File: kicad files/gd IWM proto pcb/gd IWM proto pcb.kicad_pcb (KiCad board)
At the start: 2 copper layers, 93.8 x 65.4 mm, 60 parts, among them J1 DB19_4, J10 CPx_LA, J11 Addr_Main_Data, J13 Game Port, J14 CTRL2, J15 IWM-LA, J16 FDC Hdr, J17 EN, J18 CTRL1, J19 Slot_Maker, J2 DSUB19, J3 DB19_16, J4 EN, J5 EN, J6 PWR, J8 555_LA, U1 NE556, U2 NE556, U3 IWM, U4 HCT251

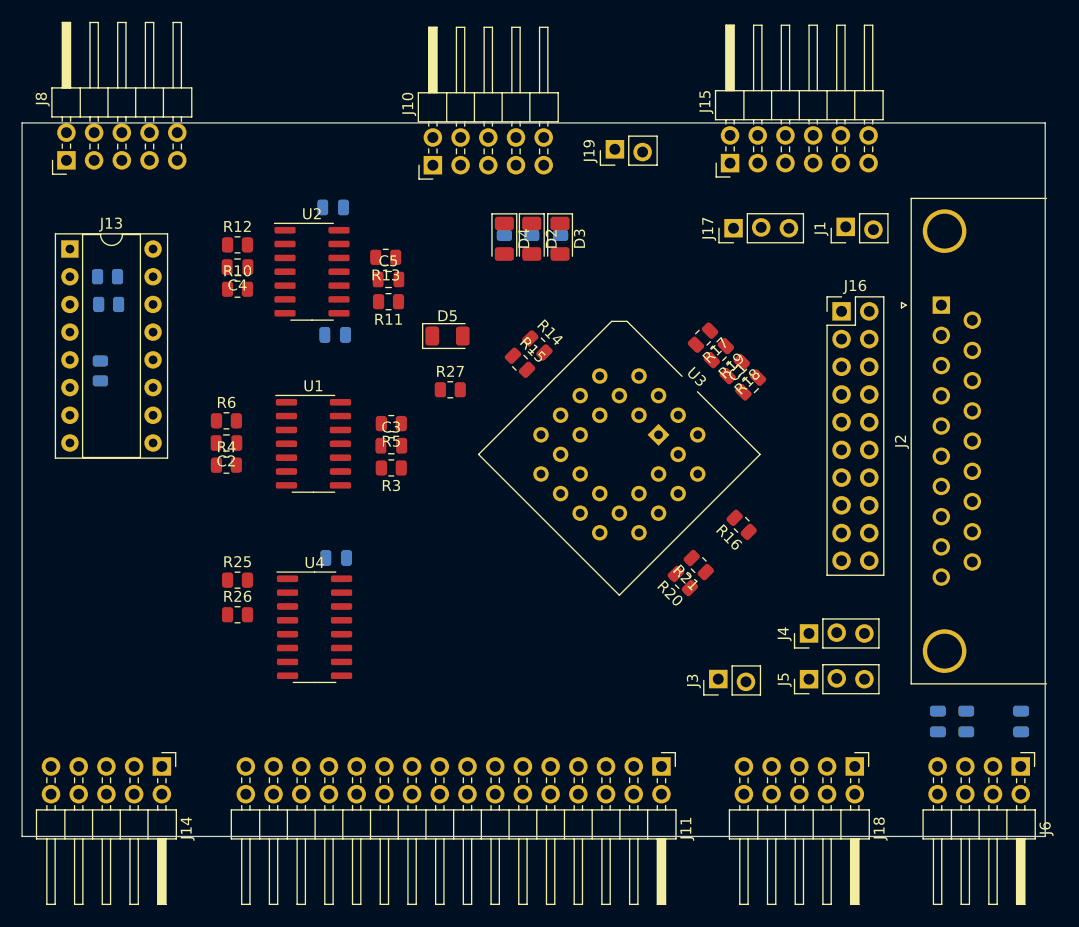
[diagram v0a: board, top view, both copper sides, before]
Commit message: routed most of critical signals. now trying to get LA headers
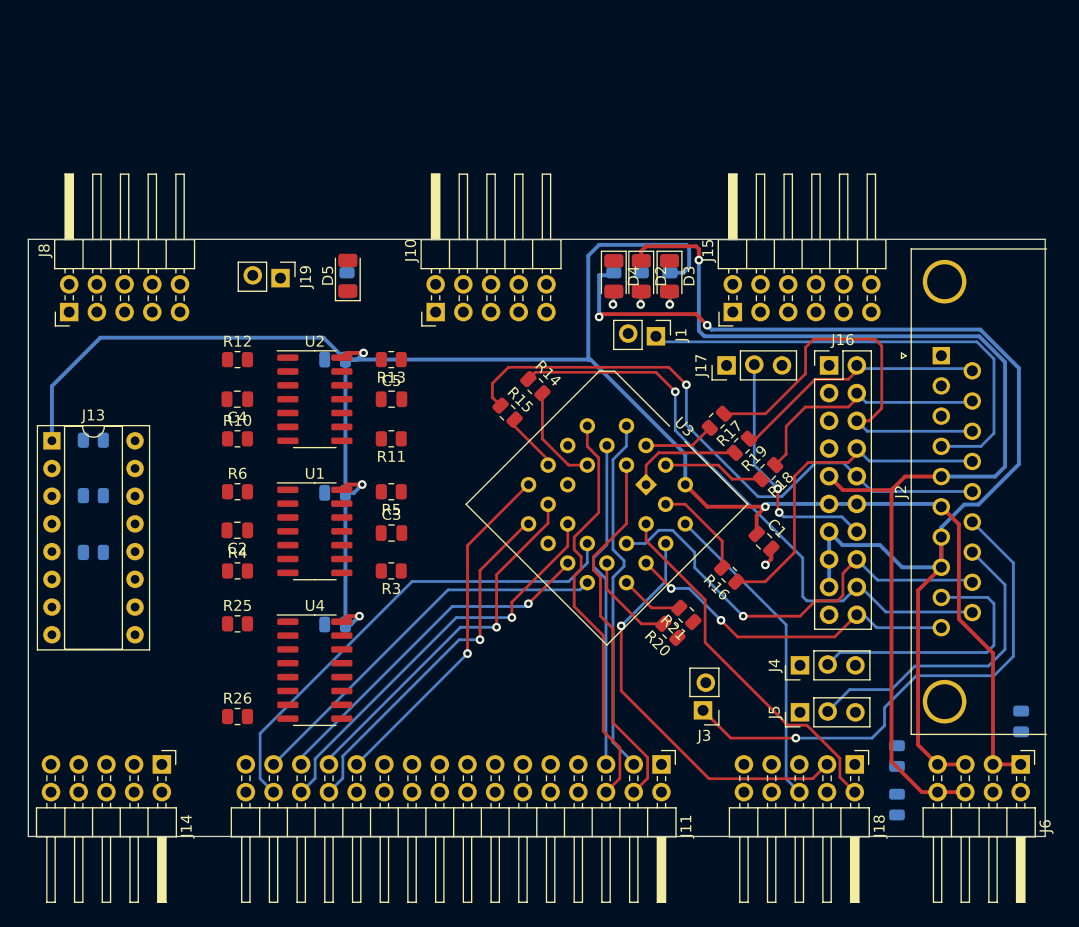
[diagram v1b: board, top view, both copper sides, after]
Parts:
- R27: moved to B.Cu
- moved J19 32.8 mm to (130.4, 81.7), turned to 270 degrees
- moved J1 20.0 mm to (164.8, 87.0), turned to 270 degrees
- moved J13 17.7 mm to (109.5, 96.7)
- moved R23 17.6 mm to (113.3, 101.7)
- moved R22 16.6 mm to (113.3, 106.9), turned to 180 degrees
- moved R24 15.0 mm to (113.3, 96.6)
- moved C9 14.5 mm to (135.4, 101.5)
- moved C1 14.4 mm to (174.8, 105.9), turned to 315 degrees
- moved C10 13.9 mm to (135.4, 89.3)
- moved J8 13.9 mm to (111.1, 84.9)
- moved R10 13.7 mm to (126.5, 96.5)
- moved J15 13.7 mm to (171.9, 84.9)
- moved R27 13.6 mm to (136.5, 82.2), turned to 90 degrees
- moved J10 13.5 mm to (144.7, 84.9)
- moved J17 12.6 mm to (171.3, 89.8)
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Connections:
- J2 pad 16: /DB19-4 -> /DB19-16
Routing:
- net +5V: track 0.00 -> 186.3 mm, vias 0 -> 4
- net +12V: track 0.00 -> 109.6 mm, vias 0 -> 2
- net -12V: track 0.00 -> 103.2 mm, vias 0 -> 1
- net /bWREQ: track 0.00 -> 56.4 mm, vias 0 -> 1
- net /bWDATA: track 0.00 -> 55.4 mm, vias 0 -> 1
- net /DB19-16: track 0.00 -> 47.5 mm, vias 0 -> 1
- net /MD6: track 0.00 -> 44.1 mm
- net /DB19-4: track 0.00 -> 44.0 mm
- net /RDATA: track 0.00 -> 40.5 mm, vias 0 -> 1
- net /seek2: track 0.00 -> 38.4 mm
- net /RESET: track 0.00 -> 37.9 mm, vias 0 -> 1
- net /BA2: track 0.00 -> 37.7 mm
- net /MD4: track 0.00 -> 37.7 mm, vias 0 -> 1
- net /MD7: track 0.00 -> 35.7 mm
- net /MD3: track 0.00 -> 34.1 mm, vias 0 -> 1
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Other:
- board size 93.8 x 65.4 mm -> 93.2 x 54.7 mm
- net class Power added: clearance 0.1524, trace_width 0.3556, via_dia 0.8, via_drill 0.4
